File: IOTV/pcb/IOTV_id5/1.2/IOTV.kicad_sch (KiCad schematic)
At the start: 23 parts, among them J1 Screw_Terminal_01x02, J2 Screw_Terminal_01x02, J3 Conn_01x04, J4 Conn_01x04, J5 Conn_01x04, J6 Conn_01x05, J8 UART, SW1 RST, SW2 Boot, U1 ESP32-WROOM-E, U2 G7DA-28 (Z)D3 8A/240V (3-32V)

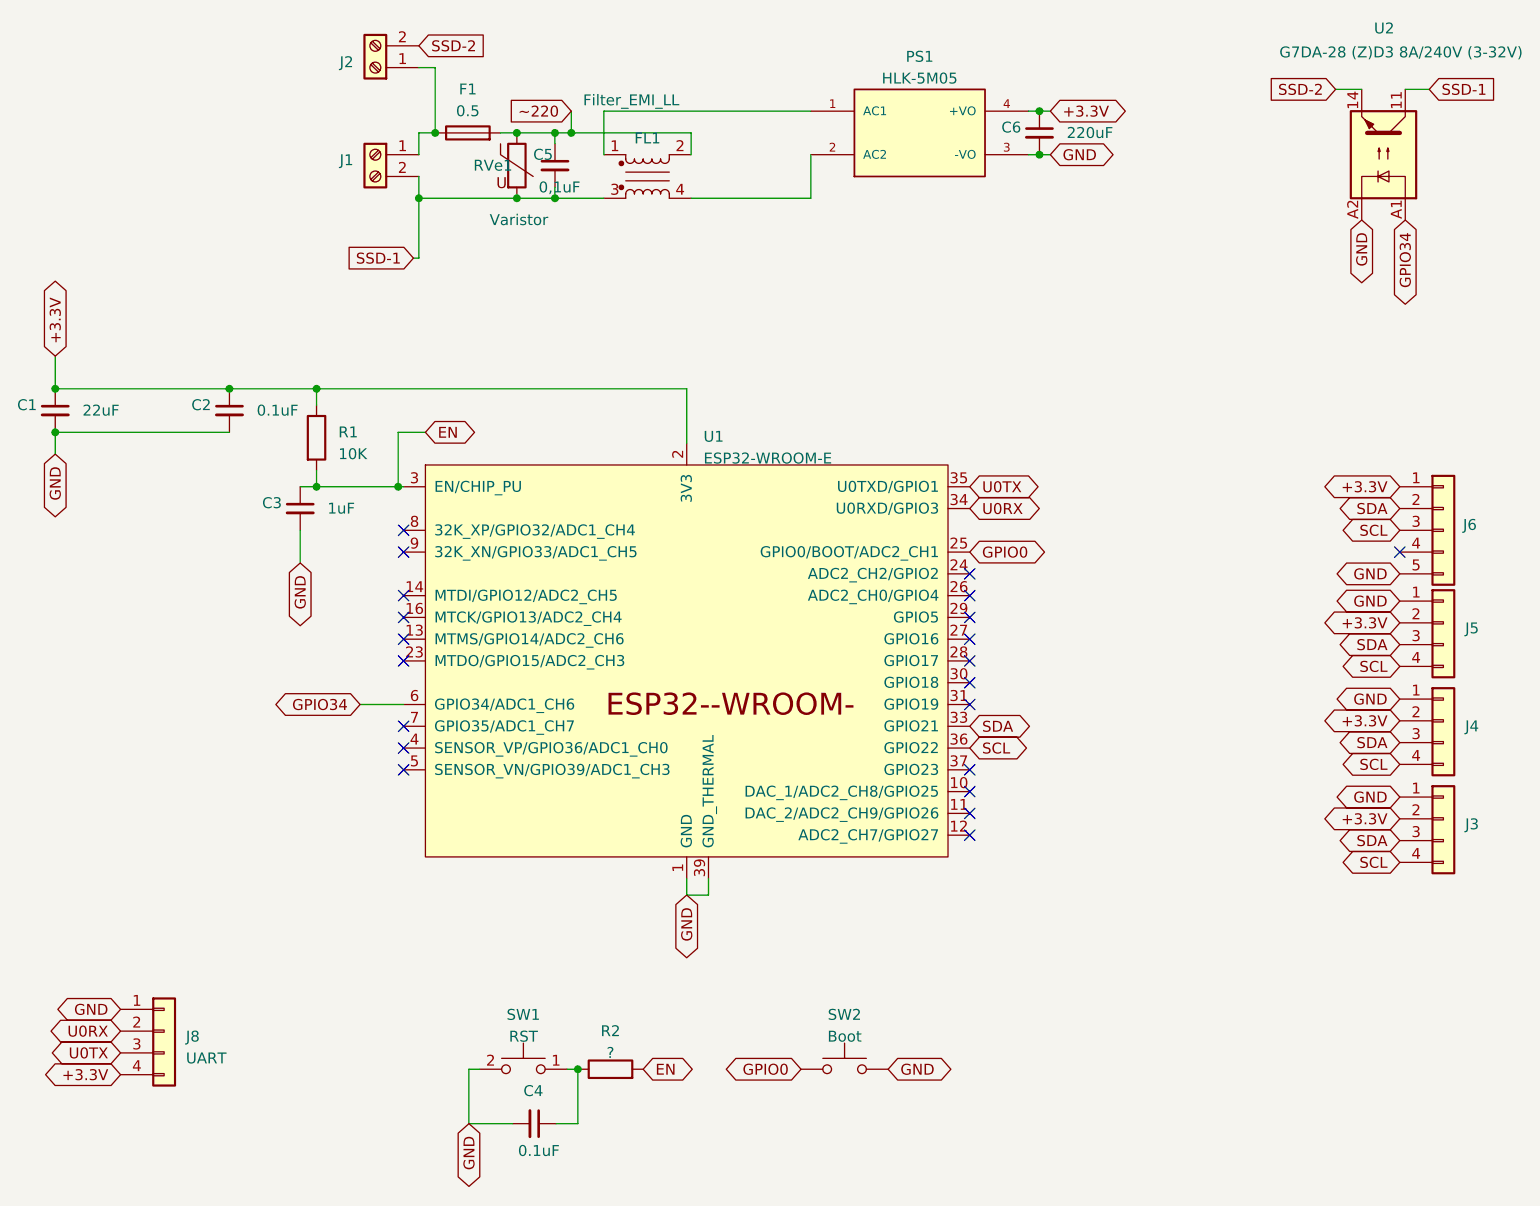
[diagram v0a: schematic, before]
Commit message: pcb id5 rev 1.2
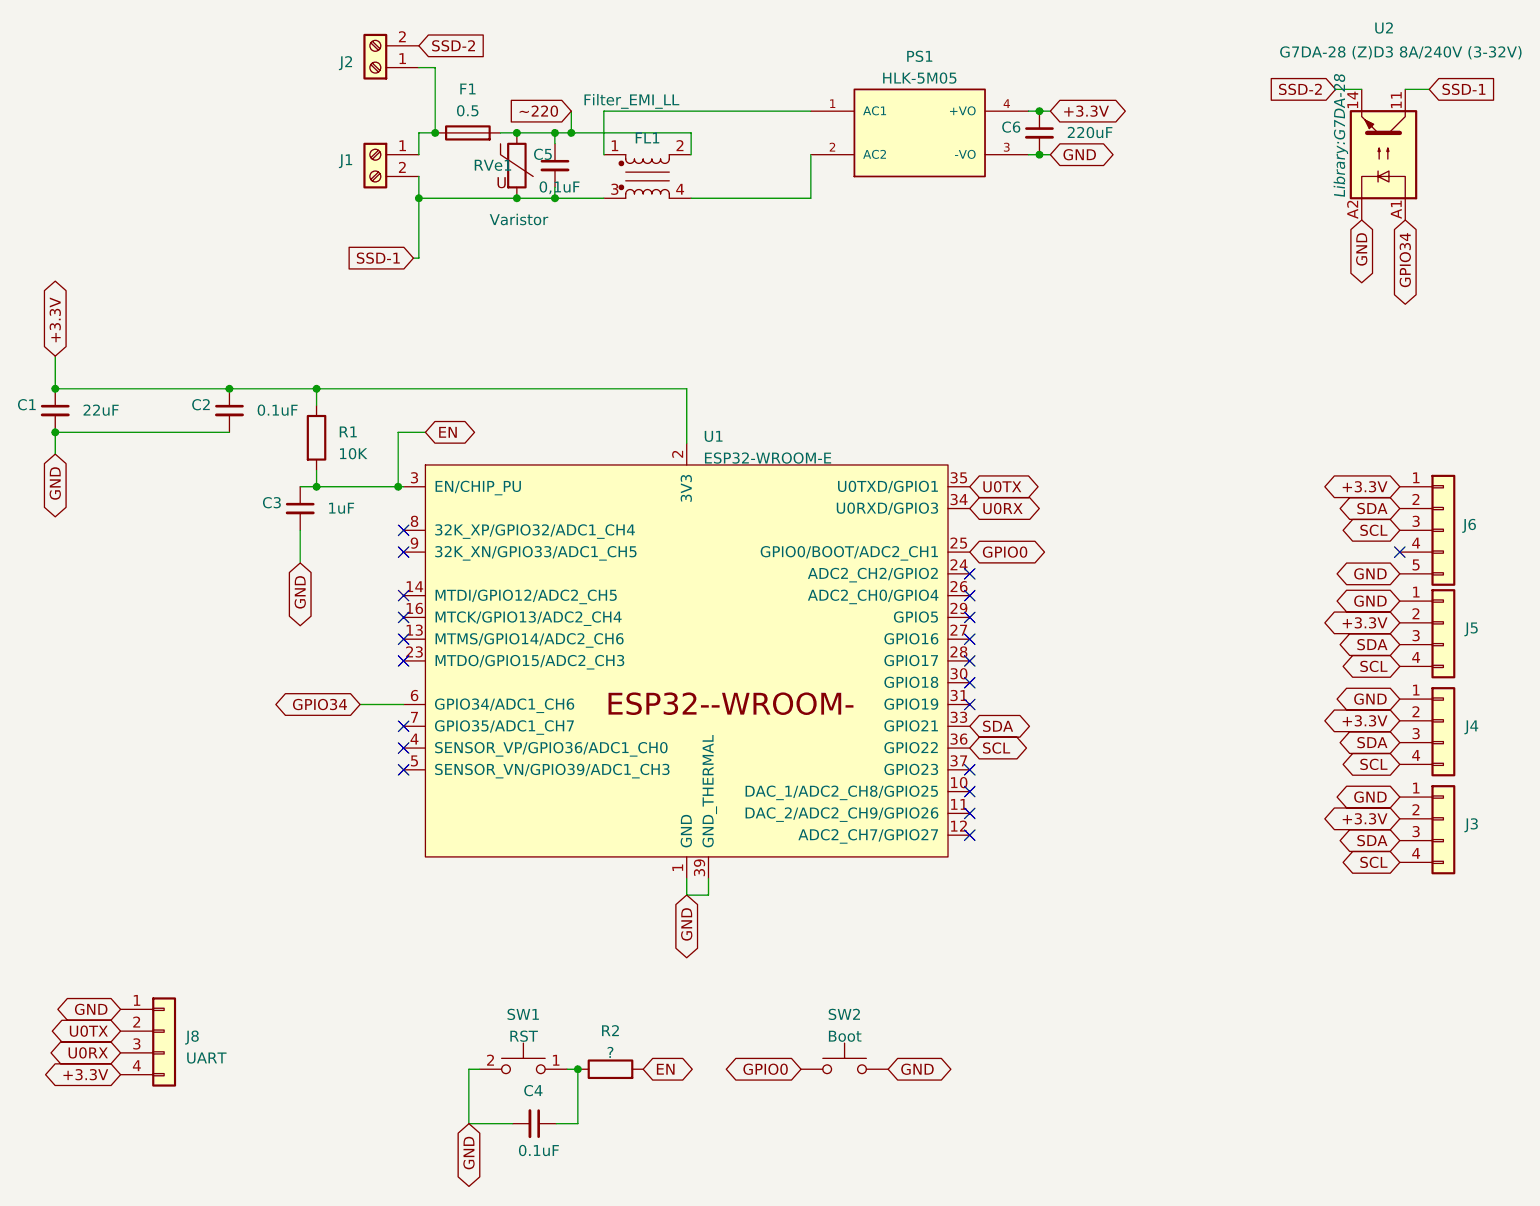
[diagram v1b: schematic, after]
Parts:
- U2: footprint OptoDevice:Finder_34.81 -> Library:G7DA-28
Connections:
- net U0RX: now also J8.3 (Pin_3); no longer J8.2 (Pin_2)
- net U0TX: now also J8.2 (Pin_2); no longer J8.3 (Pin_3)
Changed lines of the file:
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@@
     )
   )
-  (global_label "U0TX" (shape bidirectional) (at 43.18 144.145 180) (fields_autoplaced)
-    (effects (font (size 1.27 1.27)) (justify right))
-    (property "Intersheetrefs" "${INTERSHEET_REFS}" (at 34.4458 144.145 0)
+  (global_label "U0TX" (shape bidirectional) (at 43.18 141.605 180) (fields_autoplaced)
+    (effects (font (size 1.27 1.27)) (justify right))
+    (property "Intersheetrefs" "${INTERSHEET_REFS}" (at 34.4458 141.605 0)
       (effects (font (size 1.27 1.27)) (justify right))
     )
@@
     )
   )
-  (global_label "U0RX" (shape bidirectional) (at 43.18 141.605 180) (fields_autoplaced)
-    (effects (font (size 1.27 1.27)) (justify right))
-    (property "Intersheetrefs" "${INTERSHEET_REFS}" (at 34.1434 141.605 0)
+  (global_label "U0RX" (shape bidirectional) (at 43.18 144.145 180) (fields_autoplaced)
+    (effects (font (size 1.27 1.27)) (justify right))
+    (property "Intersheetrefs" "${INTERSHEET_REFS}" (at 34.1434 144.145 0)
       (effects (font (size 1.27 1.27)) (justify right))
     )
@@
       (effects (font (size 1.27 1.27)) (justify right))
     )
-    (property "Footprint" "OptoDevice:Finder_34.81" (at 185.42 44.45 0)
-      (effects (font (size 1.27 1.27) italic) (justify left) hide)
+    (property "Footprint" "Library:G7DA-28" (at 185.42 44.45 0)
+      (effects (font (size 1.27 1.27) italic) (justify left))
     )
     (property "Datasheet" "http://www.us.liteon.com/downloads/LTV-817-827-847.PDF" (at 190.5 39.37 0)
